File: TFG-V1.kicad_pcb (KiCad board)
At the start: 2 copper layers, 50.9 x 74.4 mm, 69 parts, among them CN1 1n, CN2 1n, CN3 1n, CN4 1n, CN5 1n, J1 Input, U1 AMS1117-3.3, U10 TPS72325, U11 TPD4E1U06, U12 CRE1S0505SC, U14 ESP32-C3-DevKitC-02, U15 ADuM3151, U2 TPD4E1U06, U3 ADS1298PAG, U4 TPD4E1U06, U5 LM2664, U6 MIC5504-2.5YM5, U7 TPD4E1U06, U8 TPD4E1U06, U9 TPD4E1U06

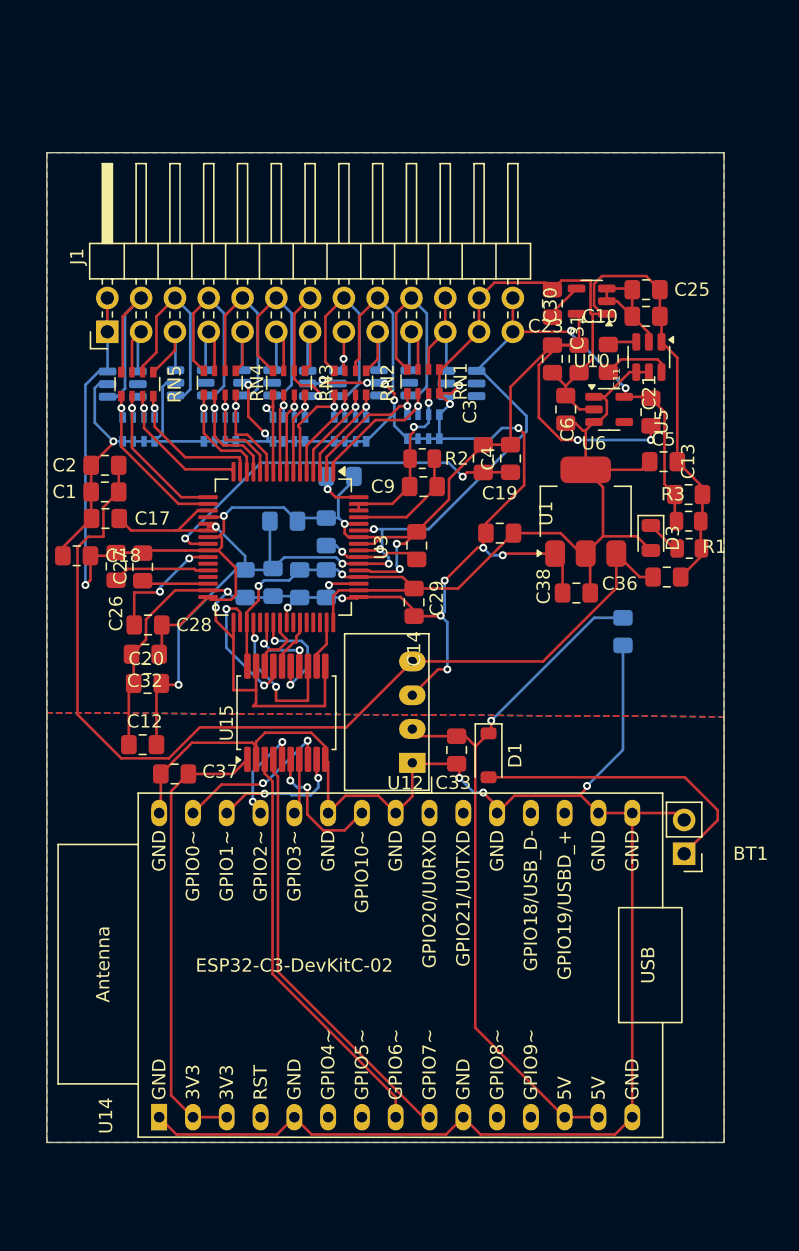
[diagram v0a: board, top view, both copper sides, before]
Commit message: arreglo1
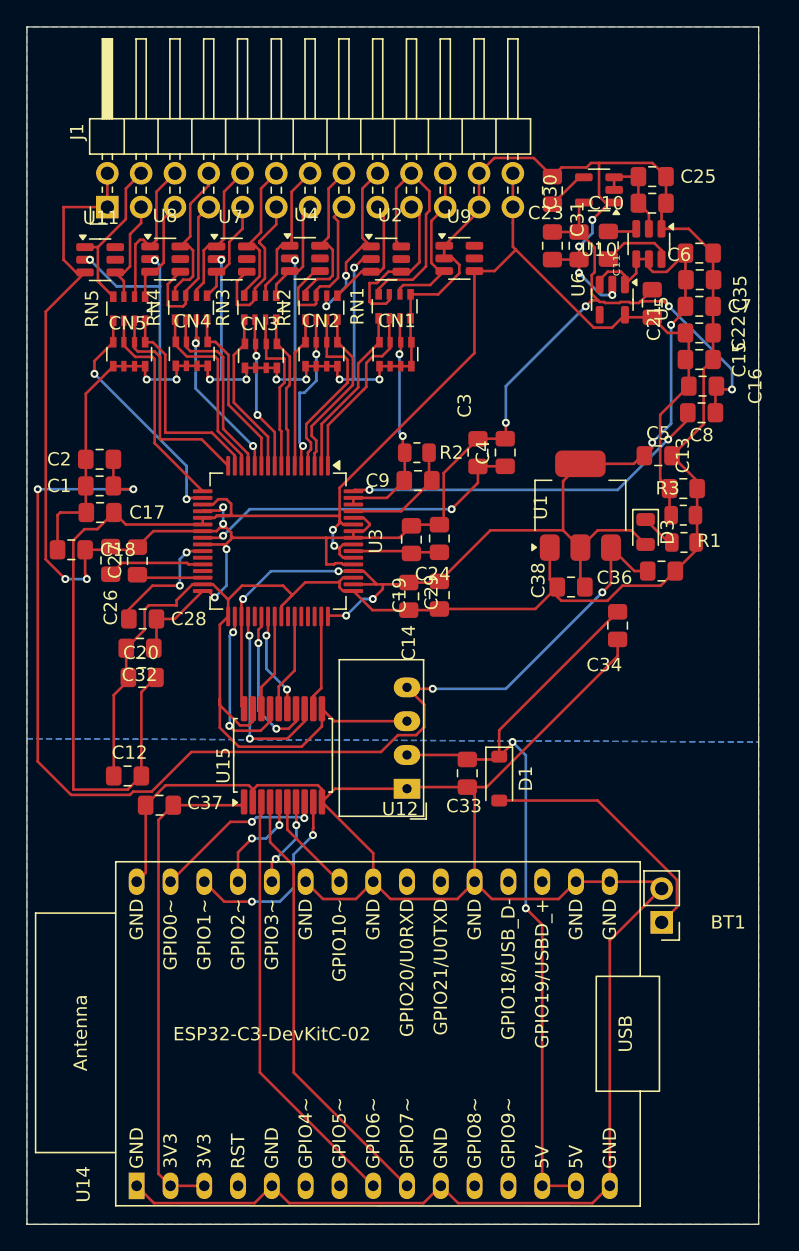
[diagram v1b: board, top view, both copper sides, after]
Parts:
- C15, C16, C22, C24, C34, C35, C7, C8, CN1, CN2, CN3, CN4, CN5, U11, U2, U4, U7, U8, U9: moved to F.Cu
- moved C15 38.1 mm to (153.0, 57.2), turned to 0 degrees
- moved C22 37.1 mm to (153.0, 55.2), turned to 0 degrees
- moved C7 36.6 mm to (153.0, 53.2), turned to 0 degrees
- moved C35 36.2 mm to (153.1, 51.2), turned to 0 degrees
- moved C16 33.1 mm to (153.3, 59.2)
- moved C8 27.6 mm to (153.2, 61.2)
- moved C6 15.5 mm to (153.0, 49.2), turned to 0 degrees
- moved U11 9.50 mm to (108.0, 49.8)
- moved U4 9.50 mm to (123.4, 49.6)
- moved U7 9.49 mm to (117.9, 49.7)
- moved U8 9.49 mm to (112.9, 49.7)
- moved U9 9.40 mm to (135.0, 49.6)
- moved J1 9.38 mm to (108.5, 45.8)
- moved U2 9.32 mm to (129.5, 49.7)
- moved C24 8.51 mm to (133.5, 70.7)
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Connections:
- CN1 pad 1: /IN_8P -> GNDD
- CN1 pad 2: /IN_8N -> GNDD
- CN1 pad 3: /IN_RLD_DRV -> GNDD
- CN1 pad 6: GNDD -> /IN_RLD_DRV
- CN1 pad 7: GNDD -> /IN_8N
- CN1 pad 8: GNDD -> /IN_8P
- CN2 pad 1: /IN_6P -> GNDD
- CN2 pad 2: /IN_6N -> GNDD
- CN2 pad 3: /IN_7P -> GNDD
- CN2 pad 4: /IN_7N -> GNDD
- CN2 pad 5: GNDD -> /IN_7N
- CN2 pad 6: GNDD -> /IN_7P
- CN2 pad 7: GNDD -> /IN_6N
- CN2 pad 8: GNDD -> /IN_6P
- CN3 pad 1: /IN_4P -> GNDD
- CN3 pad 2: /IN_4N -> GNDD
- CN3 pad 3: /IN_5P -> GNDD
- CN3 pad 4: /IN_5N -> GNDD
- CN3 pad 5: GNDD -> /IN_5N
- CN3 pad 6: GNDD -> /IN_5P
- CN3 pad 7: GNDD -> /IN_4N
- CN3 pad 8: GNDD -> /IN_4P
- CN4 pad 1: /IN_2P -> GNDD
- CN4 pad 2: /IN_2N -> GNDD
- CN4 pad 3: /IN_3P -> GNDD
- CN4 pad 4: /IN_3N -> GNDD
- CN4 pad 5: GNDD -> /IN_3N
- CN4 pad 6: GNDD -> /IN_3P
- CN4 pad 7: GNDD -> /IN_2N
- CN4 pad 8: GNDD -> /IN_2P
- CN5 pad 1: /IN_TESTP2 -> GNDD
- CN5 pad 2: /IN_TESTP1 -> GNDD
- CN5 pad 3: /IN_1P -> GNDD
- CN5 pad 4: /IN_1N -> GNDD
- CN5 pad 5: GNDD -> /IN_1N
- CN5 pad 6: GNDD -> /IN_1P
- CN5 pad 7: GNDD -> /IN_TESTP1
- CN5 pad 8: GNDD -> /IN_TESTP2
- RN1 pad 1: GNDD -> /IN_8P
- RN1 pad 2: /RLD_DRV -> /IN_8N
- RN1 pad 3: /8N -> /IN_RLD_DRV
- RN1 pad 4: /8P -> GNDD
- RN1 pad 5: /IN_8P -> GNDD
- RN1 pad 6: /IN_8N -> /RLD_DRV
- RN1 pad 7: /IN_RLD_DRV -> /8N
- RN1 pad 8: GNDD -> /8P
- RN2 pad 1: /7N -> /IN_6P
- RN2 pad 2: /7P -> /IN_6N
- RN2 pad 3: /6N -> /IN_7P
- RN2 pad 4: /6P -> /IN_7N
- RN2 pad 5: /IN_6P -> /7N
- RN2 pad 6: /IN_6N -> /7P
- RN2 pad 7: /IN_7P -> /6N
- RN2 pad 8: /IN_7N -> /6P
- RN3 pad 1: /5N -> /IN_4P
- RN3 pad 2: /5P -> /IN_4N
- RN3 pad 3: /4N -> /IN_5P
- RN3 pad 4: /4P -> /IN_5N
- RN3 pad 5: /IN_4P -> /5N
- RN3 pad 6: /IN_4N -> /5P
- RN3 pad 7: /IN_5P -> /4N
- RN3 pad 8: /IN_5N -> /4P
- RN4 pad 1: /3N -> /IN_2P
- RN4 pad 2: /3P -> /IN_2N
- RN4 pad 3: /2N -> /IN_3P
- RN4 pad 4: /2P -> /IN_3N
- RN4 pad 5: /IN_2P -> /3N
- RN4 pad 6: /IN_2N -> /3P
- RN4 pad 7: /IN_3P -> /2N
- RN4 pad 8: /IN_3N -> /2P
- RN5 pad 1: /1N -> /IN_TESTP2
- RN5 pad 2: /1P -> /IN_TESTP1
- RN5 pad 3: /TESTP1 -> /IN_1P
- RN5 pad 4: /TESTP2 -> /IN_1N
- RN5 pad 5: /IN_TESTP2 -> /1N
- RN5 pad 6: /IN_TESTP1 -> /1P
- RN5 pad 7: /IN_1P -> /TESTP1
- RN5 pad 8: /IN_1N -> /TESTP2
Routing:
- net GNDD: track 237.2 -> 276.5 mm, vias 20 -> 17
- net GND: track 133.4 -> 159.0 mm, vias 3 -> 0
- net VDDA: track 104.1 -> 128.6 mm, vias 8 -> 2
- net Net-(U3-WCT): track 3.59 -> 27.9 mm, vias 1 -> 2
- net VSSA: track 124.5 -> 146.2 mm, vias 7 -> 10
- net /5V_ISO: track 73.9 -> 91.8 mm, vias 0 -> 4
- net VDD: track 76.2 -> 91.0 mm, vias 2 -> 6
- net /6N: track 4.70 -> 13.6 mm, vias 1 -> 0
- net /8N: track 5.99 -> 12.3 mm
- net /2N: track 6.09 -> 12.3 mm
- net /4N: track 6.18 -> 12.3 mm
- net +5V: track 54.0 -> 60.1 mm, vias 1 -> 2
- net /IN_7P: track 7.90 -> 13.9 mm, vias 1 -> 0
- net /FE_START_ISO: track 5.78 -> 11.7 mm
- net /IN_5P: track 6.83 -> 12.6 mm, vias 1 -> 0
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- removed copper zone on F.Cu, net +5V
- removed copper zone on F.Cu, net VSSA
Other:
- board size 50.9 x 74.4 mm -> 55 x 90 mm
